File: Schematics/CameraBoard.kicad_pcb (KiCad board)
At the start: 2 copper layers, 81.4 x 67.8 mm, 63 parts, among them J1 Runcam Split 4 v2, J2 USB_C_Receptacle, J4 Runcam Split 4 v2, J5 Runcam Split 4 v2, SW1 SW_Push, SW2 SW_Push, U1 STM32F405RGTx, U2 TPS22917DBVR, U3 TPS22917DBVR, U4 SN65HVD230DR, U5 AMS1117-3.3, U6 TPS22917DBVR

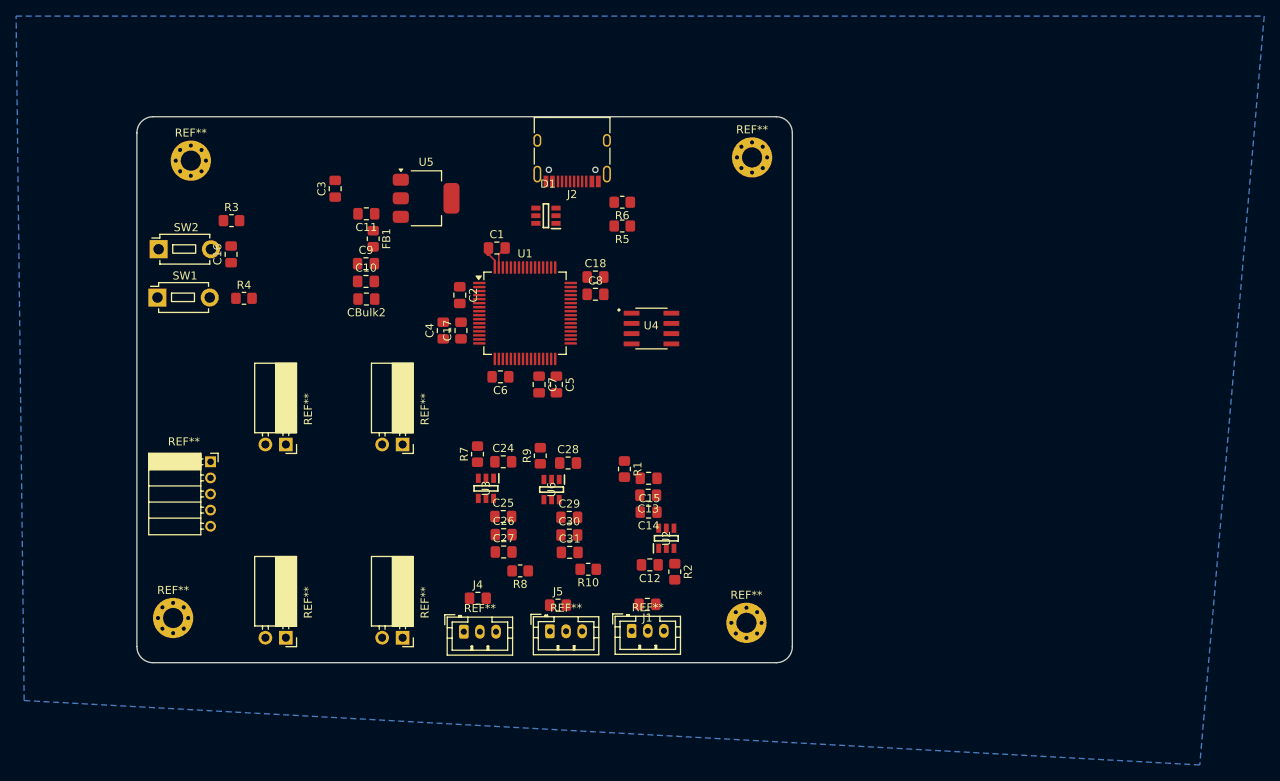
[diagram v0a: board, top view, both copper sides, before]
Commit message: fixed spacing issues
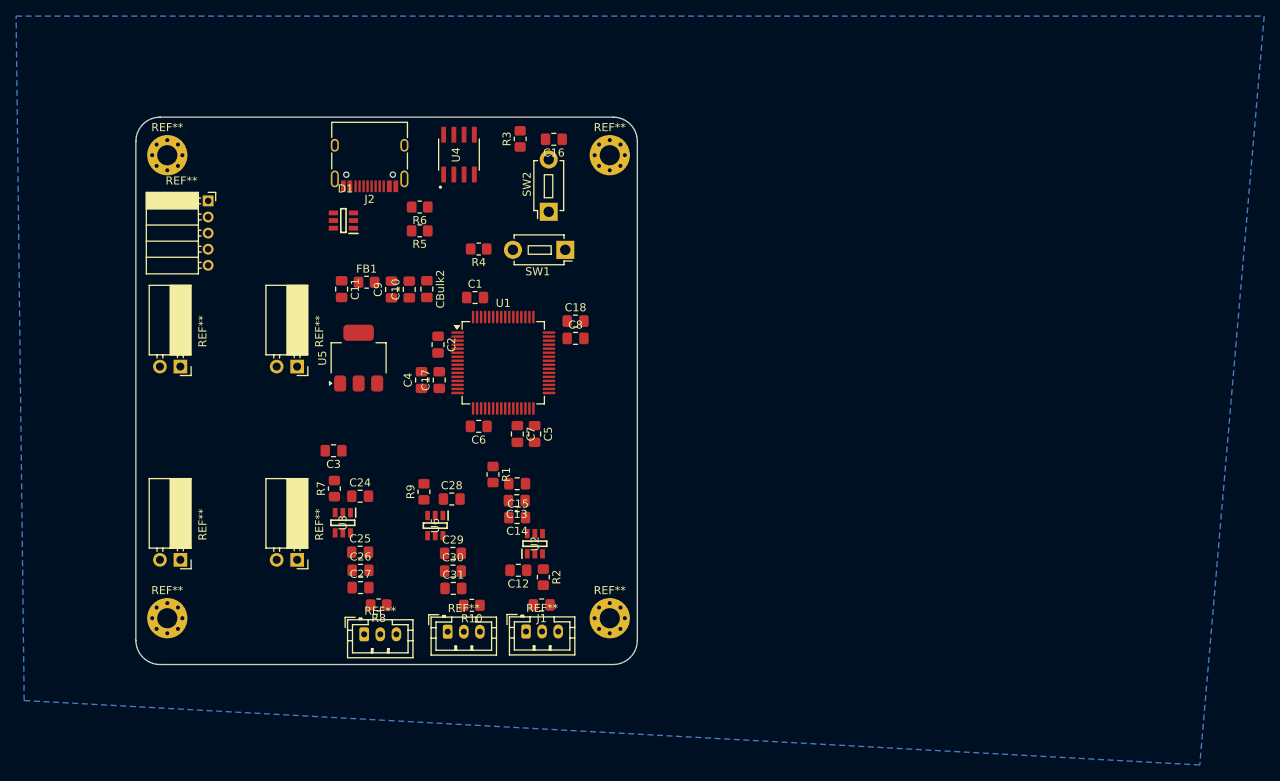
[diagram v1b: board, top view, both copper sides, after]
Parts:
- removed J4, J5: Runcam Split 4 v2, Capacitor_SMD:C_0805_2012Metric_Pad1.18x1.45mm_HandSolder
- moved SW1 51.0 mm to (105.7, 61.5), turned to 180 degrees
- moved SW2 48.7 mm to (103.7, 56.8), turned to 90 degrees
- moved C16 42.6 mm to (104.3, 47.8), turned to 180 degrees
- moved R3 37.3 mm to (100.1, 47.8), turned to 90 degrees
- moved C3 32.5 mm to (76.9, 86.5), turned to 180 degrees
- moved REF** 32.4 mm to (61.4, 55.5)
- moved U4 32.2 mm to (92.5, 49.7), turned to 90 degrees
- moved R4 29.8 mm to (95.0, 61.4), turned to 180 degrees
- moved R5 25.2 mm to (87.6, 59.2)
- moved R6 25.2 mm to (87.6, 56.2)
- moved D1 25.2 mm to (78.2, 57.9)
- moved J2 25.2 mm to (81.4, 49.6)
- moved U5 21.5 mm to (80.0, 75.0), turned to 90 degrees
- moved C25 18.3 mm to (80.2, 99.1)
- moved C26 18.3 mm to (80.3, 101.3)
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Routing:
- net +3.3V: track 3.23 -> 0.22 mm
- net GND: track 2.75 -> 0.00 mm
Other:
- board size 81.4 x 67.8 mm -> 62.3 x 68 mm
